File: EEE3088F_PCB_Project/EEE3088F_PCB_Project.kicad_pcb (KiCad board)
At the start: 2 copper layers, 6 parts, among them IC1 DRV8833PWPR, IC2 DRV8833PWPR, IC3 TPS62067DSGR, IC4 TPS62067DSGR, IC5 INA219AIDCNR, J1 Conn_02x16_Odd_Even

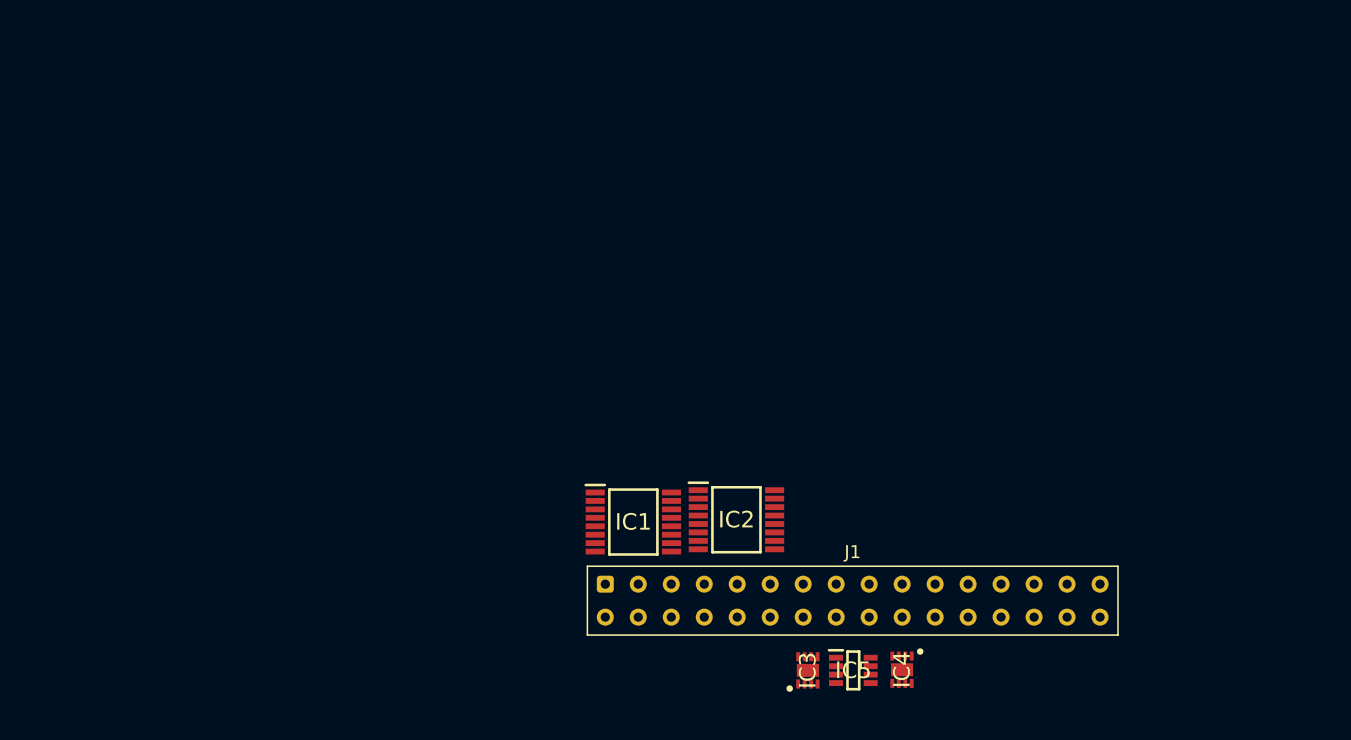
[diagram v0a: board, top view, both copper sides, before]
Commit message: v1.2
Starting with PCB design
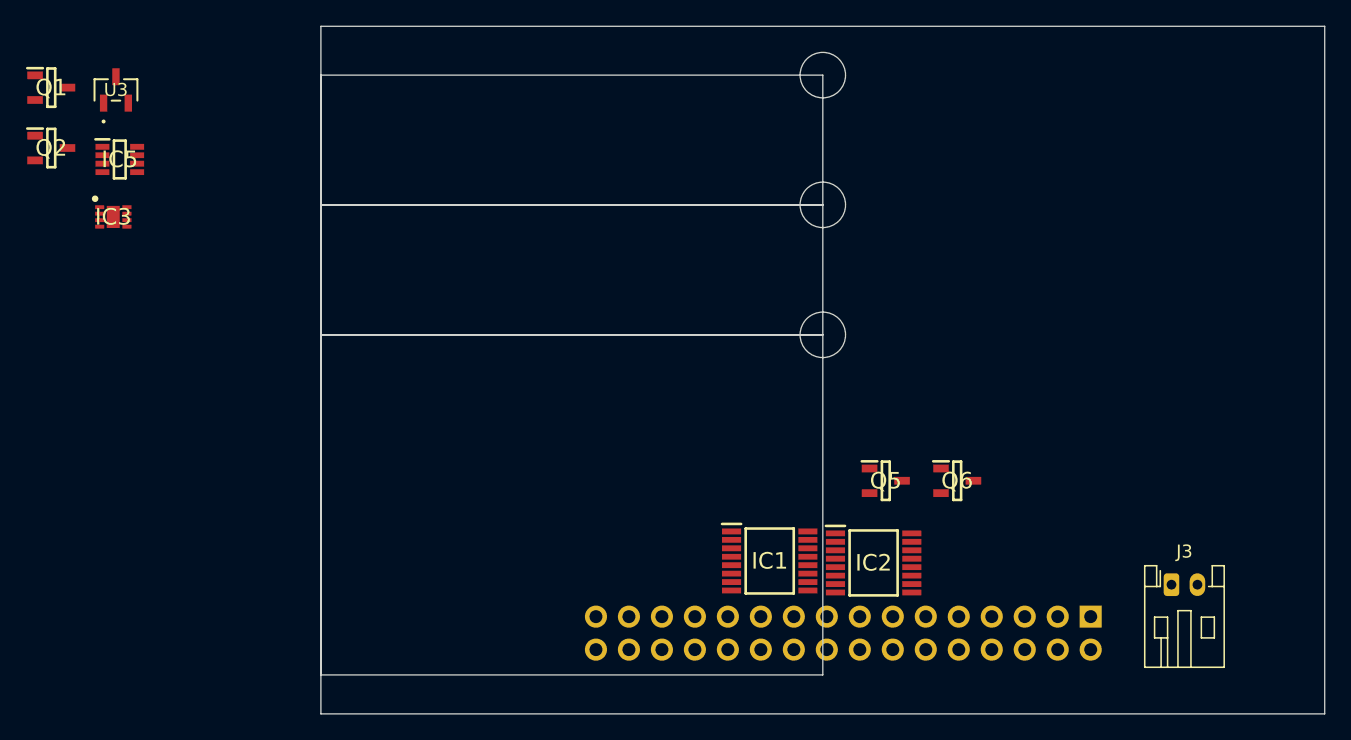
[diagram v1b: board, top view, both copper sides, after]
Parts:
- removed IC4: TPS62067DSGR, TPS62067DSGR KiCad:SON50P200X200X80-9N
- added J3: Conn_01x02, Connector_JST:JST_PH_S2B-PH-K_1x02_P2.00mm_Horizontal, F.Cu at (165.5, 96.0)
- added Q1: AO3400A, AO3400A KiCad:SOT95P280X125-3N, F.Cu at (79.2, 57.7)
- added Q2: AO3400A, AO3400A KiCad:SOT95P280X125-3N, F.Cu at (79.2, 62.4)
- added Q5: AO3401A, AO3400A KiCad:SOT95P280X125-3N, F.Cu at (143.5, 88.0)
- added Q6: AO3401A, AO3400A KiCad:SOT95P280X125-3N, F.Cu at (149.0, 88.0)
- added U3: IRLML6344TRPBF, IRLML6344TRPBF:IRLML6344TRPBF_INF, F.Cu at (84.2, 57.9)
- J1: footprint Connector_Samtec_HLE_THT:Samtec_HLE-116-02-xx-DV-TE_2x16_P2.54mm_Horizontal -> Connector_PinSocket_2.54mm:PinSocket_2x16_P2.54mm_Vertical; moved to B.Cu
- moved IC5 68.8 mm to (84.5, 63.3)
- moved IC3 63.9 mm to (84.0, 67.7), turned to 0 degrees
- moved J1 37.5 mm to (159.3, 98.5), turned to 90 degrees
- moved IC2 11.1 mm to (142.6, 94.3)
- moved IC1 10.9 mm to (134.6, 94.2)
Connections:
- IC3 pad 5: /BATTERY -> Net-(IC3-AVIN)
- IC3 pad 6: GND -> /PWR SWITCH OUT
- IC3 pad 7: /BATTERY -> Net-(IC3-AVIN)
- IC3 pad 8: /BATTERY -> Net-(IC3-AVIN)
- IC5 pad 4: /3V3 OUT -> Net-(IC5-VS)
- J1 pad 15: /RESV -> unconnected-(J1-Pin_15-Pad15)
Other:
- board outline added: 77.3 x 53 mm
